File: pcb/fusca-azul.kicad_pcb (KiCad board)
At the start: 2 copper layers, 56.5 x 65.2 mm, 12 parts, among them J3 HC-SR04, J4 L298N Logic Jumpers, J5 HC-SR04, J6 HC-SR04, U2 ESP32 - HW-394

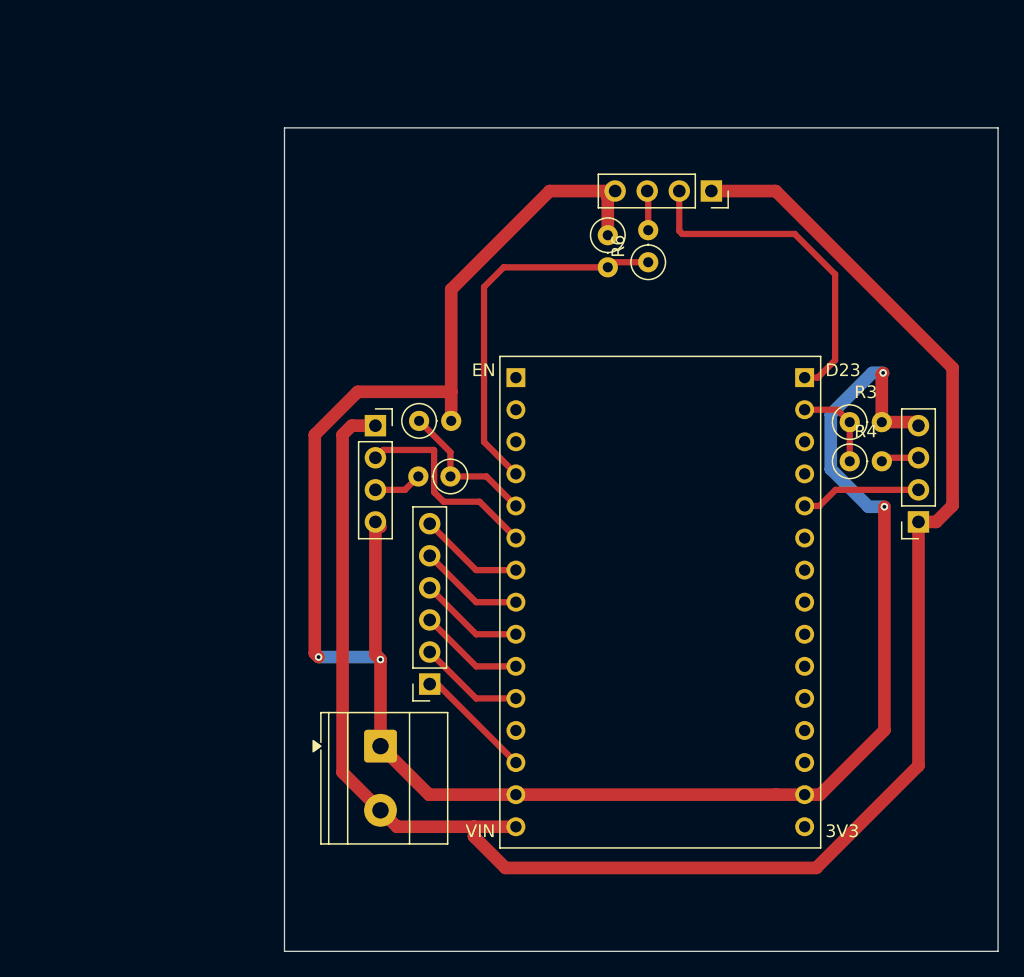
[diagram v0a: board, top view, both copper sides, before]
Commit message: feat: finaliza pcb
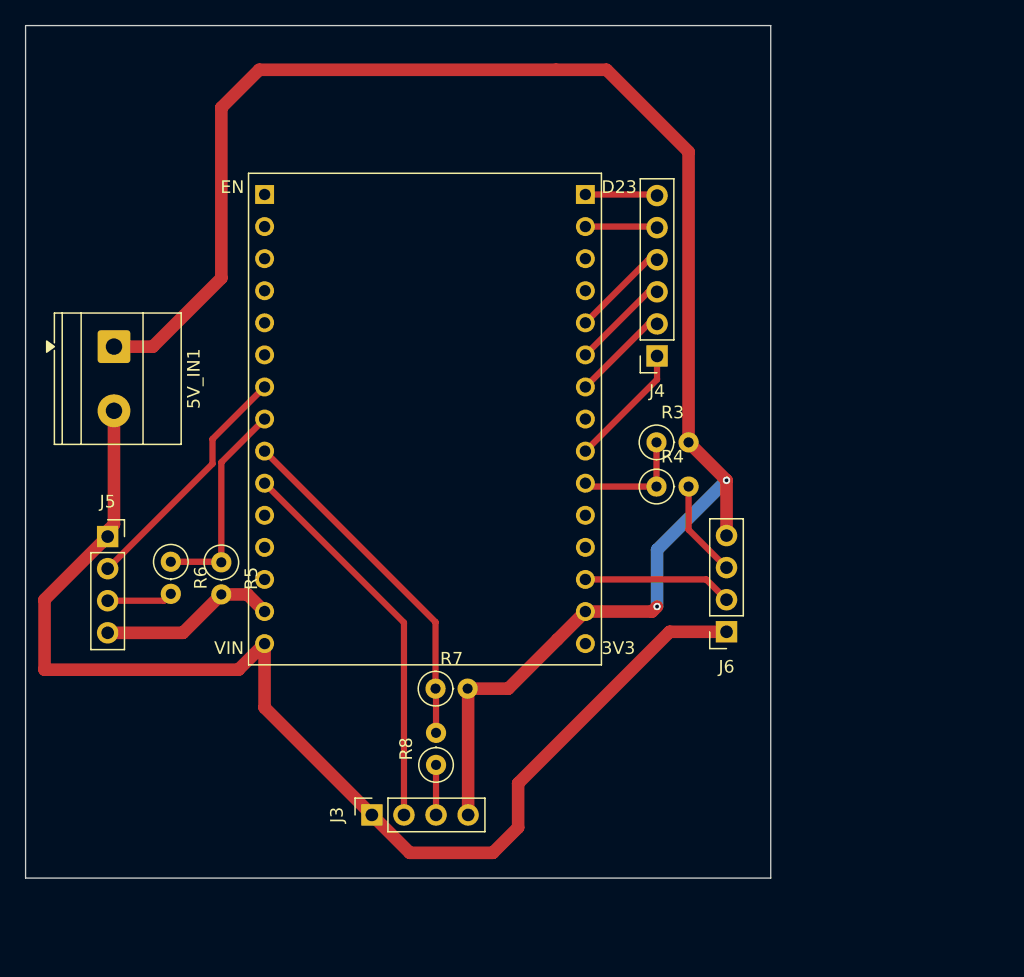
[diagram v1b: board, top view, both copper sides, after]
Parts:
- moved J5 55.1 mm to (86.5, 88.0), turned to 0 degrees
- moved J3 49.1 mm to (107.4, 110.0), turned to 90 degrees
- moved R6 44.6 mm to (91.5, 90.0), turned to -90 degrees
- moved R5 40.1 mm to (95.5, 90.0)
- moved 5V_IN1 38.0 mm to (87.0, 72.9)
- moved J6 32.2 mm to (135.5, 95.5), turned to 180 degrees
- moved J4 31.6 mm to (130.0, 73.7)
- moved U2 24.6 mm to (98.9, 60.9)
- moved R8 22.9 mm to (112.5, 106.0), turned to 90 degrees
- moved R7 21.2 mm to (112.5, 100.0)
- moved R4 15.4 mm to (130.0, 84.0)
- moved R3 15.4 mm to (130.0, 80.5)
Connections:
- J3 pad 2: Net-(J3-Trig) -> unconnected-(J3-Trig-Pad2)
- R3 pad 1: Net-(U2-D22) -> Net-(U2-RX2)
- R4 pad 1: Net-(U2-D22) -> Net-(U2-RX2)
- R4 pad 2: Net-(J3-Echo) -> Net-(J6-Echo)
- R5 pad 1: GND -> Net-(U2-D25)
- R5 pad 2: Net-(U2-D34) -> GND
- R6 pad 1: Net-(U2-D34) -> Net-(U2-D25)
- R7 pad 1: Net-(U2-D35) -> Net-(R7-Pad1)
- R8 pad 1: Net-(U2-D35) -> Net-(J3-Echo)
- R8 pad 2: Net-(J6-Echo) -> Net-(R7-Pad1)
- U2 pad 10: Net-(J6-Trig) -> unconnected-(U2-D32-Pad10)
- U2 pad 11: Net-(U2-D35) -> unconnected-(U2-D35-Pad11)
- U2 pad 12: Net-(U2-D34) -> unconnected-(U2-D34-Pad12)
- U2 pad 18: unconnected-(U2-D15-Pad18) -> Net-(J6-Trig)
- U2 pad 21: unconnected-(U2-RX2-Pad21) -> Net-(U2-RX2)
- U2 pad 22: unconnected-(U2-TX2-Pad22) -> Net-(J4-ENA)
- U2 pad 24: unconnected-(U2-D18-Pad24) -> Net-(J4-IN_1)
- U2 pad 25: unconnected-(U2-D19-Pad25) -> Net-(J4-IN_2)
- U2 pad 26: Net-(J3-Trig) -> Net-(J4-IN_3)
- U2 pad 29: Net-(U2-D22) -> Net-(J4-IN_4)
- U2 pad 3: Net-(J4-ENA) -> unconnected-(U2-D13-Pad3)
- U2 pad 30: Net-(J5-Trig) -> Net-(J4-ENB)
- U2 pad 5: Net-(J4-IN_1) -> unconnected-(U2-D14-Pad5)
- U2 pad 6: Net-(J4-IN_2) -> unconnected-(U2-D27-Pad6)
- U2 pad 7: Net-(J4-IN_3) -> unconnected-(U2-D26-Pad7)
- U2 pad 8: Net-(J4-IN_4) -> Net-(U2-D25)
- U2 pad 9: Net-(J4-ENB) -> Net-(J5-Trig)
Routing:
- net +5V: track 143.8 -> 96.8 mm
- net unconnected-(J3-Trig-Pad2): track 0.00 -> 30.8 mm
- net Net-(U2-D34): track 29.7 -> 0.00 mm
- net Net-(R7-Pad1): track 0.00 -> 27.9 mm
- net Net-(U2-D25): track 0.00 -> 16.8 mm
- net GND: track 167.8 -> 151.0 mm, vias 4 -> 2
- net Net-(U2-D35): track 11.6 -> 0.00 mm
- net Net-(J3-Trig): track 9.54 -> 0.00 mm
- net Net-(U2-RX2): track 0.00 -> 9.24 mm
- net Net-(J5-Trig): track 26.7 -> 19.5 mm
- net Net-(U2-D22): track 7.08 -> 0.00 mm
- net Net-(J6-Trig): track 16.2 -> 11.8 mm
- net Net-(J6-Echo): track 3.84 -> 7.66 mm
- net Net-(J4-IN_4): track 8.35 -> 5.71 mm
- net Net-(J4-ENB): track 8.35 -> 5.71 mm
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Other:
- board size 56.5 x 65.2 mm -> 59 x 67.5 mm
